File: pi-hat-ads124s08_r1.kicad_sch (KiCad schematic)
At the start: 28 parts, among them J1 GPIO, J2 Conn_01x06, J3 Conn_01x06, J4 Conn_01x06, J5 Conn_01x06, J6 Conn_01x06, J7 Conn_01x02, U1 M24c64, U3 XC6206P332MR

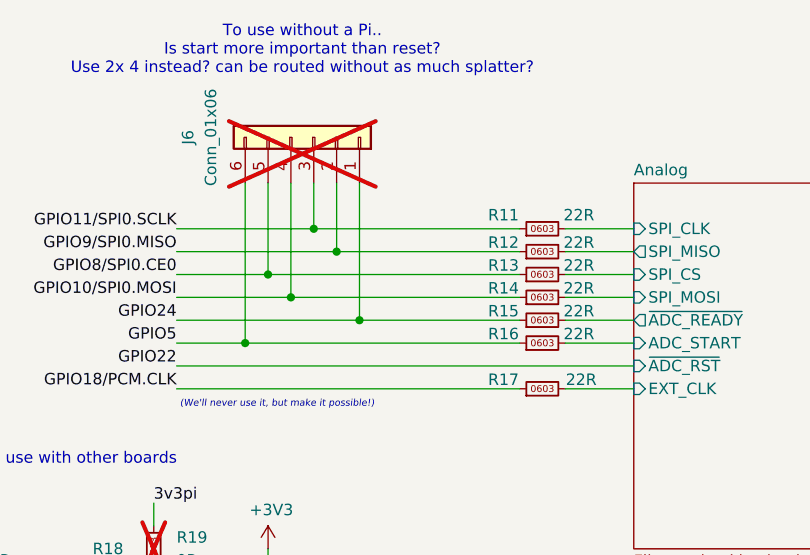
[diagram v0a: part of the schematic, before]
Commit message: thanks, I hate it.
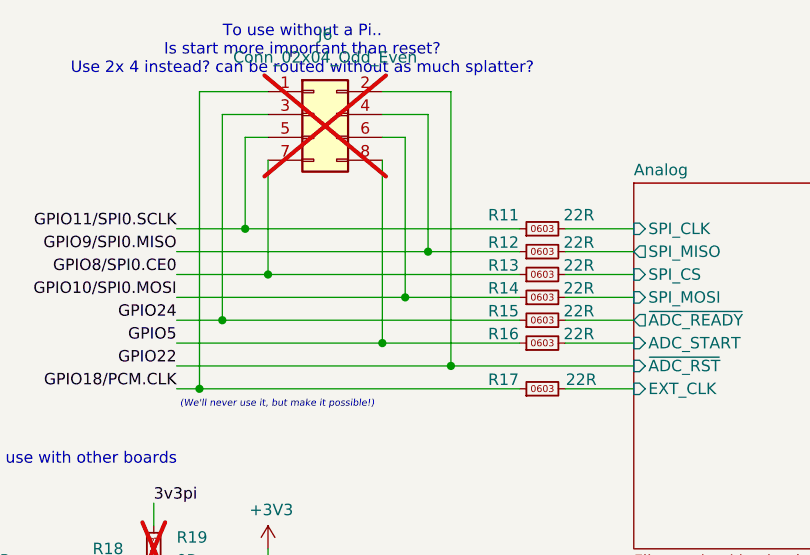
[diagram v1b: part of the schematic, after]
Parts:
- removed J6: Conn_01x06, Connector_PinHeader_2.54mm:PinHeader_1x06_P2.54mm_Vertical, symbol Connector_Generic:Conn_01x06
- added J6: Conn_02x04_Odd_Even, Connector_PinHeader_2.54mm:PinHeader_2x04_P2.54mm_Vertical, symbol Connector_Generic:Conn_02x04_Odd_Even
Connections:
- net GPIO10/SPI0.MOSI: now also J6.6 (Pin_6)
- net GPIO11/SPI0.SCLK: now also J6.5 (Pin_5)
- net GPIO18/PCM.CLK: now also J6.1 (Pin_1)
- net GPIO22: now also J6.2 (Pin_2)
- net GPIO24: now also J6.3 (Pin_3)
- net GPIO5: now also J6.8 (Pin_8)
- net GPIO8/SPI0.CE0: now also J6.7 (Pin_7)
- net GPIO9/SPI0.MISO: now also J6.4 (Pin_4)

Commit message: moarh updates
we commit to save our progress
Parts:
- JP1: footprint Jumper:SolderJumper-2_P1.3mm_Open_TrianglePad1.0x1.5mm -> jlc-extras:SolderJumper-2_P1.3mm_Open_TrianglePad0.9x1.8mm
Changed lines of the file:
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@@
 			)
 		)
-		(property "Footprint" "Jumper:SolderJumper-2_P1.3mm_Open_TrianglePad1.0x1.5mm"
+		(property "Footprint" "jlc-extras:SolderJumper-2_P1.3mm_Open_TrianglePad0.9x1.8mm"
 			(at 97.79 180.34 0)
 			(effects
